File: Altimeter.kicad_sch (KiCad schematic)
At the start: 28 parts, among them IC1 XC9801B503KR-G, IC2 ATTINY804-SSF, IC3 MC3479, IC4 MCP73855-I_MF, IC5 XC9265B181MR-G, J1 USB3075-30-A, J2 Battery, J3 Conn_01x03_Female, U1 ICP-10111

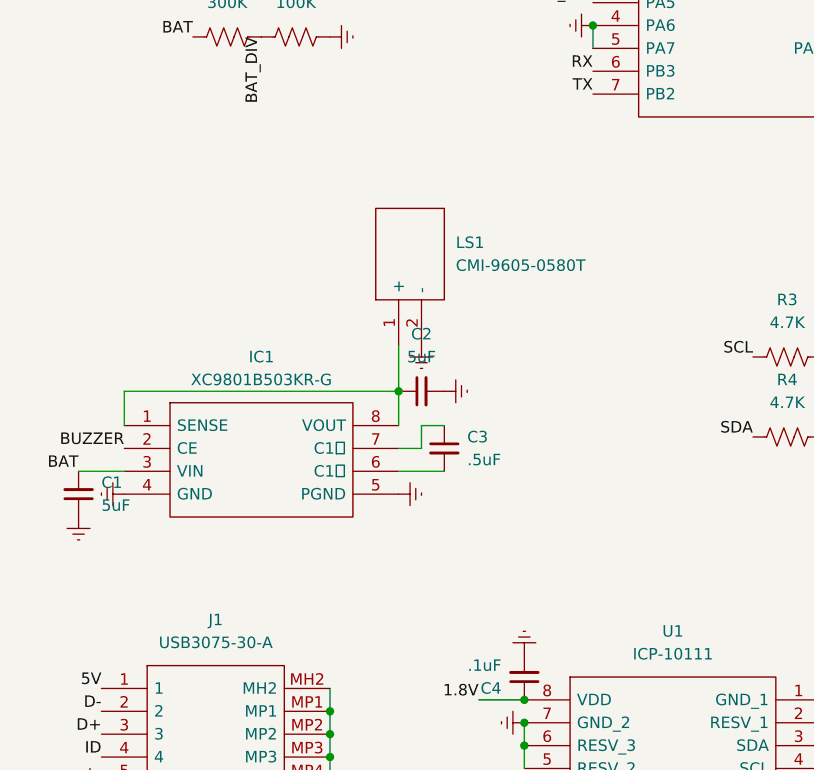
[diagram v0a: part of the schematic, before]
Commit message: changes
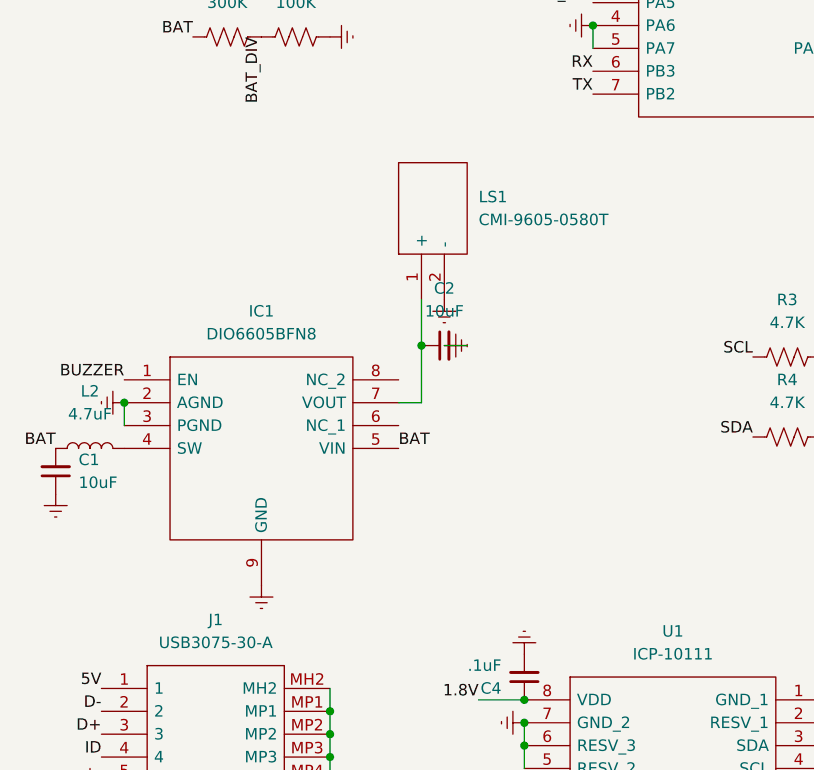
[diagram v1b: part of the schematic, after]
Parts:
- removed C3: .5uF, Capacitor_SMD:C_0805_2012Metric_Pad1.18x1.45mm_HandSolder, symbol Device:C_Small
- removed IC1: XC9801B503KR-G, SamacSys_Parts:SOP65P490X122-8N, symbol SamacSys_Parts:XC9801B503KR-G
- added IC1: DIO6605BFN8, SamacSys_Parts:SON50P300X200X80-9N-D, symbol SamacSys_Parts:DIO6605BFN8
- added L2: 4.7uF, Inductor_SMD:L_0805_2012Metric_Pad1.05x1.20mm_HandSolder, symbol Device:L
- C1, C2: value 5uF -> 10uF
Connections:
- net BAT: now also IC1.5 (VIN), L2.1
- net BUZZER: now also IC1.1 (EN)
- net Earth: now also IC1.2 (AGND), IC1.3 (PGND), IC1.9 (GND)
- net at C2.1, LS1.1 (+): now also IC1.7 (VOUT)
- new net: IC1.4 (SW), L2.2
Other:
- moved on the sheet: C1, C2, LS1
